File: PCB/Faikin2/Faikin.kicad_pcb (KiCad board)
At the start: 2 copper layers, 70 x 70 mm, 30 parts, among them J1 1x5, J3 Shelly, Q1 BSS138PS, U2 Barcode, U3 MD8942, U4 ESP32-S3-MINI-1

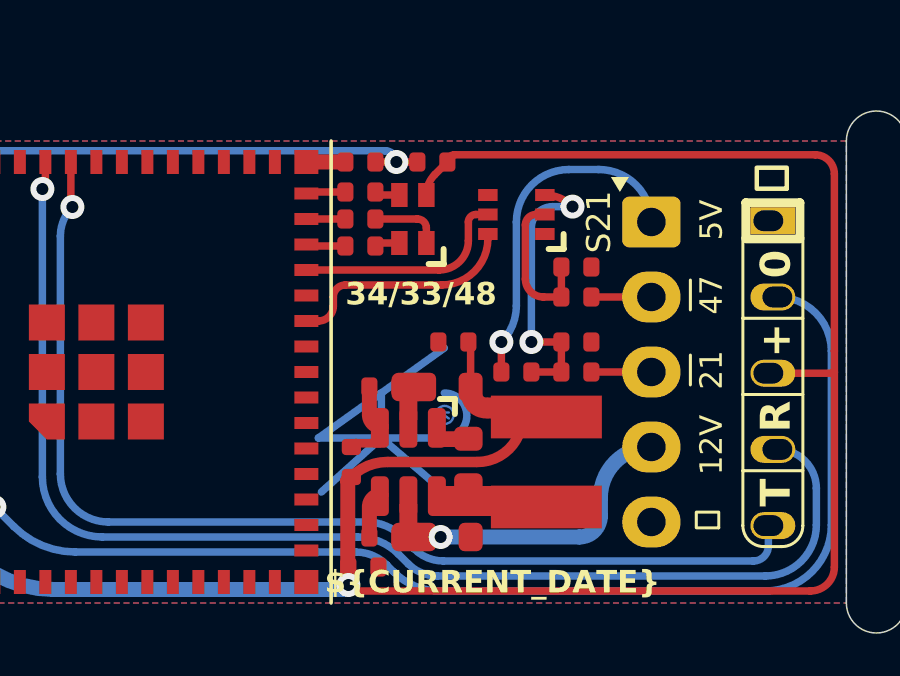
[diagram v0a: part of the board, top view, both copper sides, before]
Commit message: Silkscreen
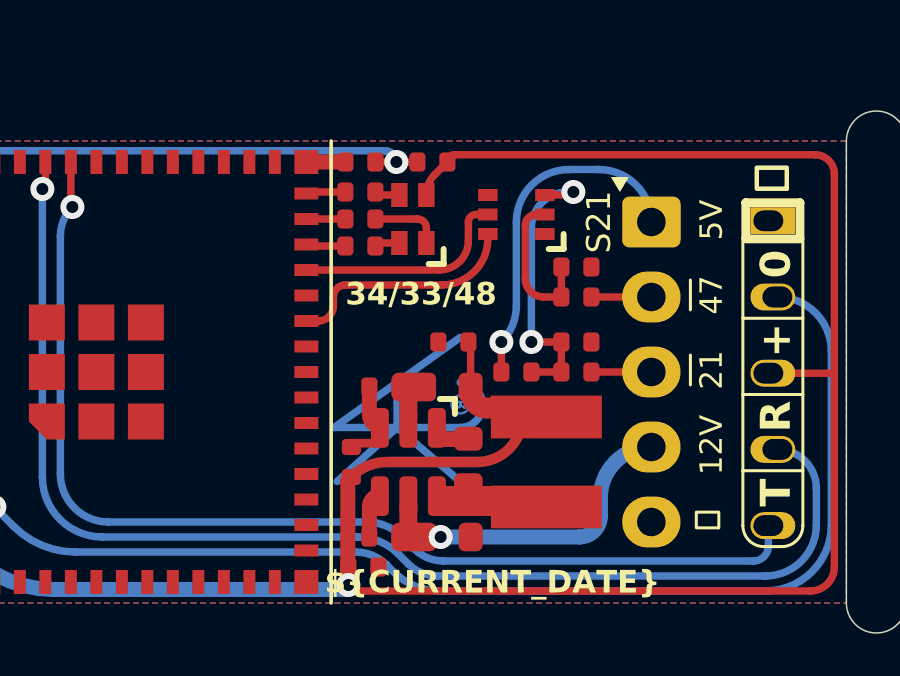
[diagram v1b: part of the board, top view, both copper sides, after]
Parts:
- moved Logo1 0.63 mm to (136.1, 62.9)
